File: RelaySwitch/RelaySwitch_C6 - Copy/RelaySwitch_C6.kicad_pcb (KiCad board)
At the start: 2 copper layers, 67.5 x 52 mm, 39 parts, among them J1 AC_MAINS_IN, J3 LOAD_CH1, J4 LOAD_CH2, J5 SW1_INPUT, J6 SW2_INPUT, K1 G5Q-1-DC5, K2 G5Q-1-DC5, Q1 MMBT8050, Q2 MMBT8050, U1 HLK-2M05, U2 XIAO-ESP32-C6-DIP, U5 HLW8012

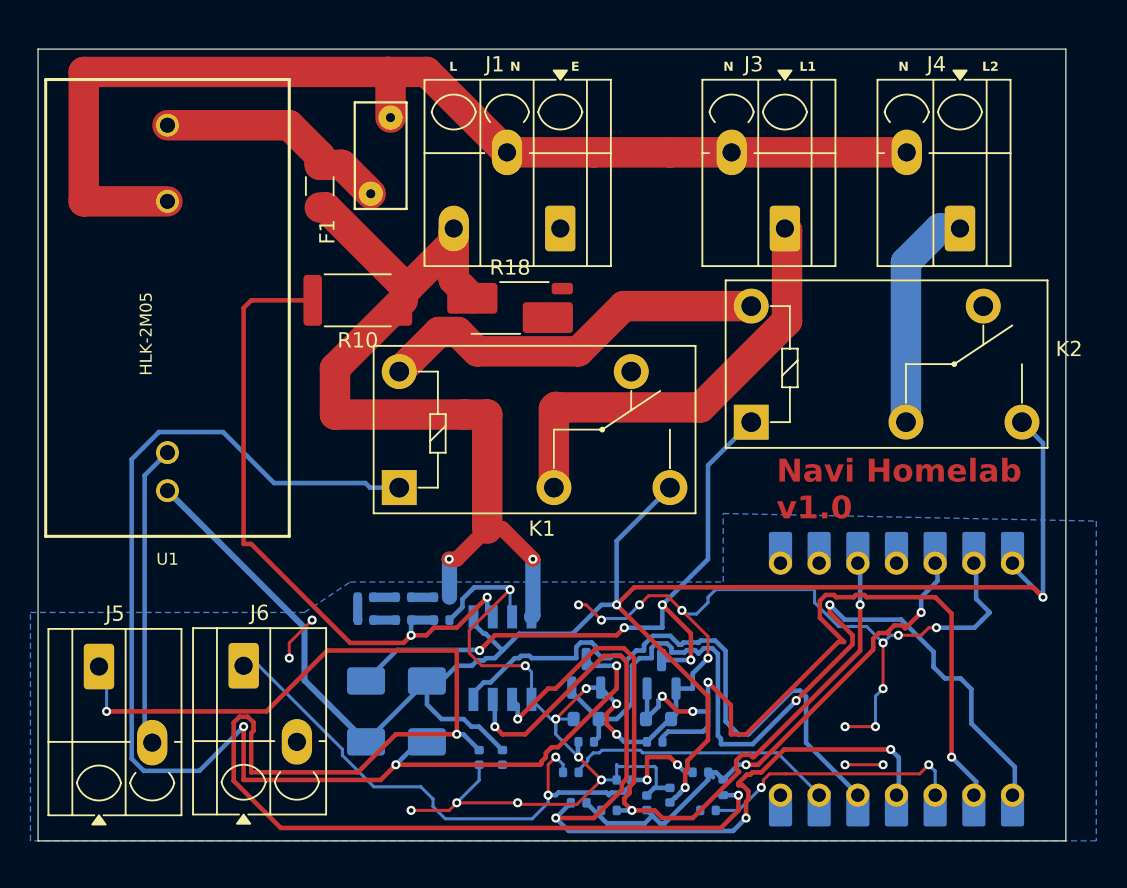
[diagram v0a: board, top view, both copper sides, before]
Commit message: For review
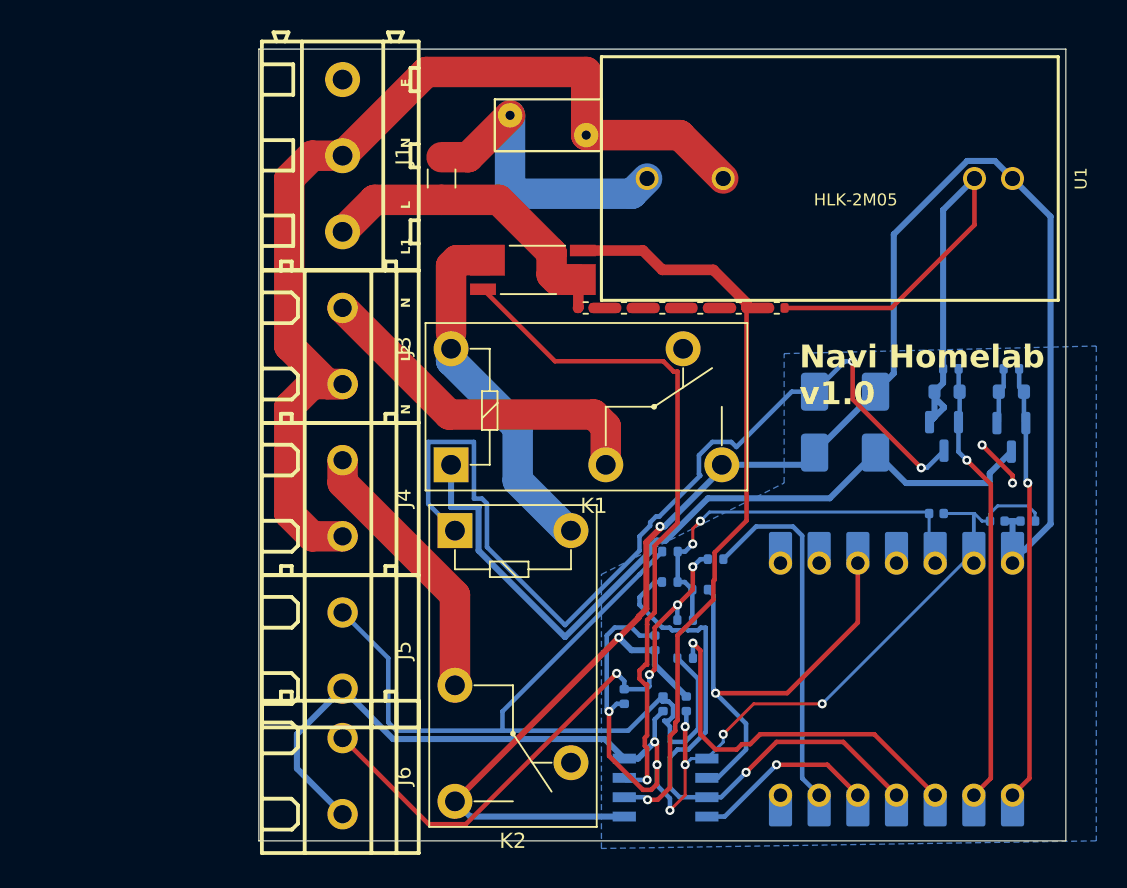
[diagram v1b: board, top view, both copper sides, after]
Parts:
- removed R10: 1m, Resistor_SMD:R_2512_6332Metric
- added C2: 10u, Capacitor_SMD:C_0402_1005Metric, B.Cu at (190.5, 80.0)
- added C3: 100n, Capacitor_SMD:C_0402_1005Metric, B.Cu at (186.5, 79.5)
- J1: footprint TerminalBlock_Degson:TerminalBlock_Degson_DG250-3.5-03P_1x03_P3.50mm_45Degree -> seeed esp32:CONN-TH_3P-P5.00_WJ128V-5.0-3P
- J3, J4, J5, J6: footprint TerminalBlock_Degson:TerminalBlock_Degson_DG250-3.5-02P_1x02_P3.50mm_45Degree -> seeed esp32:CONN-TH_2P-P5.00_WJ128V-5.0-2P
- R13, R4, R6, R7, R8, R9: moved to F.Cu
- R18: footprint Resistor_SMD:R_Shunt_Vishay_WSK2512_6332Metric_T2.66mm -> XIAO_Series_Footprints:RES_WSK2512R0100FEA
- U2: footprint XIAO_Series_Footprints:XIAO-ESP32-S3-DIP -> XIAO_Series_Footprints:XIAO-ESP32-C6-DIP
- U5: footprint XIAO_Series_Footprints:SOIC8 -> seeed esp32:SOIC8
- moved U1 44.3 mm to (179.5, 57.5), turned to 0 degrees
- moved J4 44.3 mm to (147.5, 78.5), turned to -90 degrees
- moved D1 37.8 mm to (182.5, 73.5), turned to -90 degrees
- moved R2 37.1 mm to (191.4, 70.0)
- moved R1 35.2 mm to (191.4, 71.5)
- moved D2 32.3 mm to (178.5, 73.5), turned to 90 degrees
- moved Q1 31.9 mm to (191.4, 74.5), turned to -90 degrees
- moved R5 31.3 mm to (187.4, 70.0)
- moved C5 31.1 mm to (192.5, 80.0), turned to 0 degrees
- moved R13 30.1 mm to (173.5, 66.0)
- moved R9 30.1 mm to (176.0, 66.0)
- moved J3 30.1 mm to (147.5, 68.5), turned to -90 degrees
- moved R8 30.0 mm to (171.0, 66.0)
- moved R3 28.7 mm to (187.2, 71.5), turned to 180 degrees
- moved R7 27.2 mm to (168.5, 66.0), turned to 0 degrees
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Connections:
- C5 pad 1: +3V3 -> +5V
- U5 pad 3: GND -> Net-(U5-V1N)
- U5 pad 4: /L -> GND
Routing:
- net Net-(U5-V1N): track 0.00 -> 44.9 mm, vias 0 -> 1
- net Net-(C7-Pad1): track 97.5 -> 55.3 mm, vias 3 -> 0
- net /L: track 57.7 -> 21.2 mm, vias 2 -> 0
- net Net-(D1-A): track 85.4 -> 52.0 mm, vias 3 -> 0
- net /RELAY_CH1_IN: track 58.2 -> 28.7 mm, vias 2 -> 1
- net /HLW_SEL: track 40.8 -> 12.2 mm, vias 0 -> 1
- net /RELAY_CH2_IN: track 53.6 -> 29.4 mm, vias 4 -> 1
- net /HLW_CF1: track 58.5 -> 37.6 mm, vias 4 -> 1
- net /HLW_CF: track 49.7 -> 30.1 mm, vias 3 -> 1
- net Net-(D2-A): track 43.7 -> 63.1 mm, vias 4 -> 2
- net +5V: track 123.4 -> 110.8 mm, vias 3 -> 2
- net +3V3: track 35.6 -> 26.0 mm
- net Net-(U2-GPIO2_A2_D2): track 17.6 -> 25.1 mm, vias 2 -> 1
- net Net-(U5-V1P): track 43.6 -> 51.0 mm, vias 2 -> 1
- net /MAINS_N: track 73.6 -> 67.5 mm
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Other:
- board size 67.5 x 52 mm -> 53 x 52 mm
